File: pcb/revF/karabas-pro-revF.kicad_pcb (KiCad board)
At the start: 2 copper layers, 101.6 x 147.3 mm, 240 parts, among them CON1 JOYSTICK, CON2 KEYBOARD, CON3 MOUSE, CON4 12V, CON5 SD CARD, CON6 CF CARD, CON7 SOUND, CON8 VGA, J1 FPGA JTAG, J2 I2C, J3 FDD POWER, J4 FDD, J5 TAPE IN, J6 TAPE OUT, J7 USB C, Q1 IRLML2402, Q2 IRLML2402, Q3 IRLML2402, Q4 IRLML2402, Q5 BC856, SW1 SW_SPST, U1 EP4CE22E22C8N, U10 EPM3128ATC100-10N, U11 LM2596S-5, U12 AMS1117-3.3, U13 AMS1117-2.5, U14 AMS1117-1.2, U15 74LS38, U16 74LS06, U17 MB8877A, U18 ESP-12E, U19 AMS1117-3.3, U20 LM311, U21 UDA1334ATS, U22 SN74LV1T34DBV, U3 CY62167EV30LL, U4 24LC08B, U5 W25Q128JVS, U6 DS3231MZ, U7 LM1117MP-3.3, U8 74HC597, U9 RP2040, X1 50 MHz, Y1 12MHz

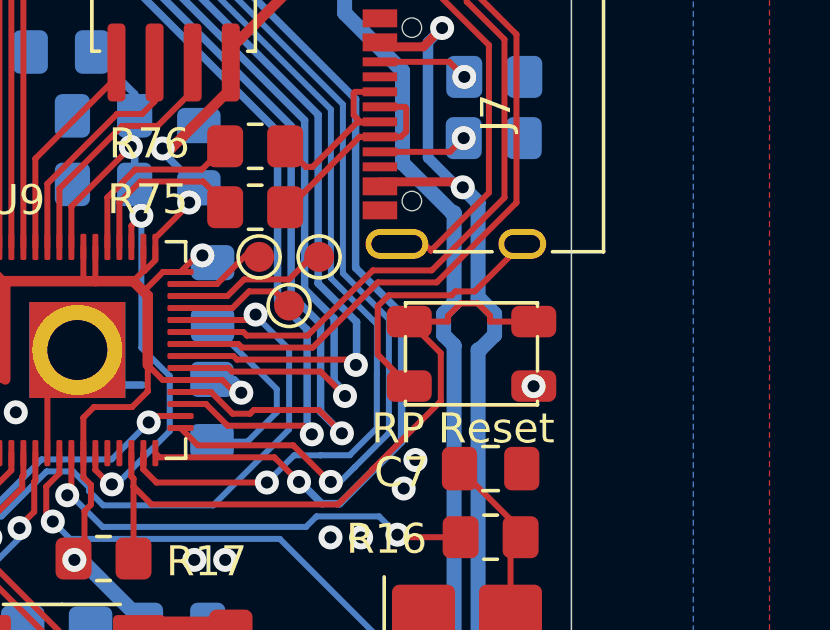
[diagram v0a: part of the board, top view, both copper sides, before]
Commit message: minor pcb revF fixes
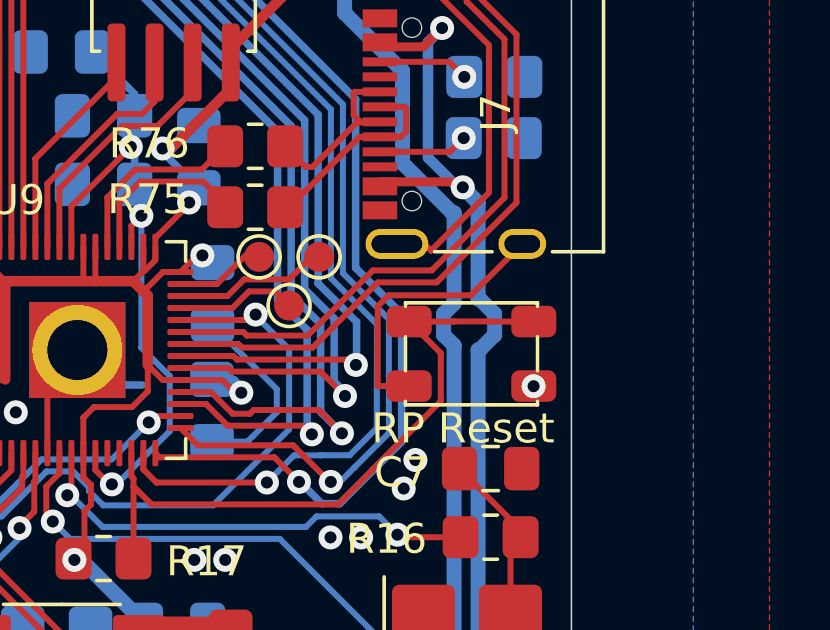
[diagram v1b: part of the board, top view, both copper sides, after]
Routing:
- net RP_RESET: track 23.4 -> 22.7 mm
- net GND: track 205.1 -> 205.7 mm
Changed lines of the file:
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@@
 	)
 	(segment
-		(start 199.0228 113.5674)
-		(end 197.4402 115.15)
-		(width 0.2)
-		(layer "F.Cu")
-		(net 1)
-	)
-	(segment
 		(start 159.568 85.797)
 		(end 159.568 88.773)
@@
 	)
 	(segment
-		(start 194.204 115.646)
-		(end 194.204 117.254)
+		(start 194.204 118.304)
+		(end 194.205 118.305)
 		(width 0.2)
 		(layer "F.Cu")
@@
 	)
 	(segment
-		(start 196.794364 115.15)
-		(end 196.664364 115.28)
-		(width 0.2)
-		(layer "F.Cu")
-		(net 1)
-	)
-	(segment
 		(start 157.808692 100.02199)
 		(end 157.818 100.031298)
@@
 	)
 	(segment
+		(start 199.0228 113.5674)
+		(end 197.3102 115.28)
+		(width 0.2)
+		(layer "F.Cu")
+		(net 1)
+	)
+	(segment
 		(start 158.04201 100.02199)
 		(end 159.004 99.06)
@@
 	)
 	(segment
+		(start 194.57 115.28)
+		(end 194.204 115.646)
+		(width 0.2)
+		(layer "F.Cu")
+		(net 1)
+	)
+	(segment
 		(start 160.568 101.147)
 		(end 160.568 99.382501)
@@
 	)
 	(segment
-		(start 196.664364 115.28)
-		(end 194.57 115.28)
-		(width 0.2)
-		(layer "F.Cu")
-		(net 1)
-	)
-	(segment
 		(start 162.663341 98.204343)
 		(end 162.663341 97.178659)
@@
 	)
 	(segment
-		(start 194.204 117.254)
+		(start 194.205 118.305)
 		(end 195.255 118.305)
 		(width 0.2)
@@
 	)
 	(segment
-		(start 197.4402 115.15)
-		(end 196.794364 115.15)
+		(start 194.204 115.646)
+		(end 194.204 118.304)
 		(width 0.2)
 		(layer "F.Cu")
@@
 	)
 	(segment
+		(start 197.3102 115.28)
+		(end 194.57 115.28)
+		(width 0.2)
+		(layer "F.Cu")
+		(net 1)
+	)
+	(segment
 		(start 129.7468 117.4672)
 		(end 128.7272 117.4672)
@@
 	)
 	(segment
-		(start 194.57 115.28)
-		(end 194.204 115.646)
-		(width 0.2)
-		(layer "F.Cu")
-		(net 1)
-	)
-	(segment
 		(start 129.7468 107.9672)
 		(end 130.572813 107.9672)
@@
 	)
 	(segment
-		(start 197.53995 115.55)
-		(end 197.95 115.96005)
+		(start 185.9923 121.3179)
+		(end 186.0644 121.39)
 		(width 0.2)
 		(layer "F.Cu")
@@
 	)
 	(segment
-		(start 195.255 116.155)
-		(end 196.55 116.155)
+		(start 197.95 116.155)
+		(end 199.405 116.155)
 		(width 0.2)
 		(layer "F.Cu")
@@
 	)
 	(segment
-		(start 185.9923 121.3179)
-		(end 186.0644 121.39)
+		(start 196.73995 116.15)
+		(end 197.945 116.15)
 		(width 0.2)
 		(layer "F.Cu")
@@
 	)
 	(segment
-		(start 196.96005 115.55)
-		(end 197.53995 115.55)
+		(start 197.945 116.15)
+		(end 197.95 116.155)
 		(width 0.2)
 		(layer "F.Cu")
@@
 	)
 	(segment
-		(start 197.95 116.155)
-		(end 199.405 116.155)
+		(start 196.73495 116.155)
+		(end 196.73995 116.15)
 		(width 0.2)
 		(layer "F.Cu")
@@
 	)
 	(segment
-		(start 197.95 115.96005)
-		(end 197.95 116.155)
-		(width 0.2)
-		(layer "F.Cu")
-		(net 20)
-	)
-	(segment
 		(start 185.9923 120.5409)
 		(end 185.9923 121.3179)
@@
 	)
 	(segment
-		(start 196.55 115.96005)
-		(end 196.96005 115.55)
+		(start 186.0644 121.39)
+		(end 186.0644 121.65)
 		(width 0.2)
 		(layer "F.Cu")
@@
 	)
 	(segment
-		(start 186.0644 121.39)
-		(end 186.0644 121.65)
+		(start 195.255 116.155)
+		(end 196.73495 116.155)
 		(width 0.2)
 		(layer "F.Cu")
@@
 		(width 0.2)
 		(layer "F.Cu")
-		(net 20)
-	)
-	(segment
-		(start 196.55 116.155)
-		(end 196.55 115.96005)
-		(width 0.2)
-		(layer "F.Cu")
